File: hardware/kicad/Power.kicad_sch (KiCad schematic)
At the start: 0 parts

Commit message: start pwr circuitry
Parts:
- added C38: 4.7uF, Diode_SMD:D_SMF, symbol Device:C
- added C39: 10uF, Diode_SMD:D_SMF, symbol Device:C
- added C40: 100nF, Diode_SMD:D_SMF, symbol Device:C
- added D29: SMF5V0A, Diode_SMD:D_SMF, symbol Diode:SMF5V0A
- added F1: Polyfuse, Package_LCC:PLCC-84_29.3x29.3mm_P1.27mm, symbol Device:Polyfuse
- added FB2: FerriteBead, symbol Device:FerriteBead
- added H1, H2, H3, H4: MountingHole_Pad, Connector_Audio:Jack_6.35mm_Neutrik_NMJ6HFD2-AU_Horizontal, symbol Mechanical:MountingHole_Pad
- added U2: LP2985-5.0, Package_TO_SOT_SMD:SOT-23-5, symbol Regulator_Linear:LP2985-5.0
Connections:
- new net: C38.1, D29.1 (A1), F1.2, FB2.1
- new net GND: C38.2, C39.2, C40.2, D29.2 (A2)
- new net SHIELD_GND: H1.1, H2.1, H3.1, H4.1
- new net USB_VBUS: C39.1, C40.1, FB2.2
- new net VBUS_RAW: F1.1
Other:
- note added: "Analog 3.3V Conversion"
- note added: "Chassis/Shield GND Conn."
- note added: "Digital 3.3V Conversion"
- note added: "USB VBUS Entry"
- company: (none) -> Jeevan Sanchez
- title: (none) -> Power Circuitry

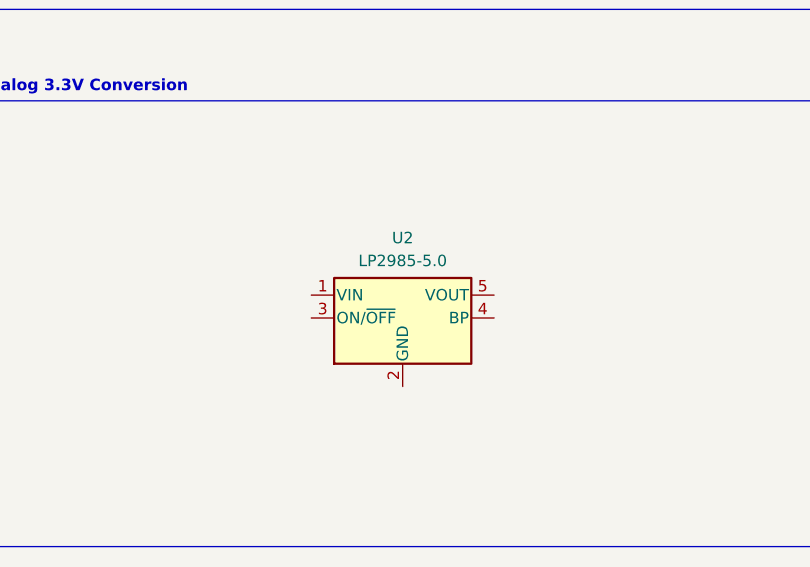
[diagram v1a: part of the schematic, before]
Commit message: ldo selection
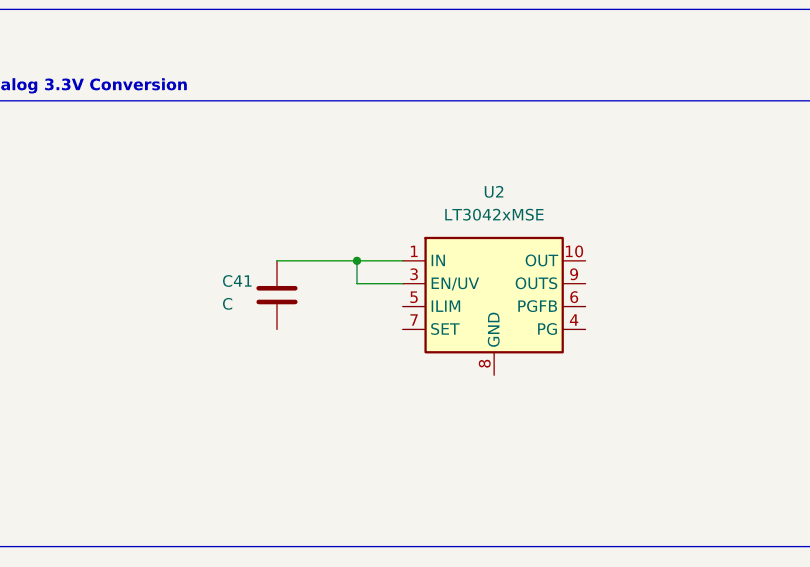
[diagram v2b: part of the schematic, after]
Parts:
- removed U2: LP2985-5.0, Package_TO_SOT_SMD:SOT-23-5, symbol Regulator_Linear:LP2985-5.0
- added C41: C, Package_SO:MSOP-10-1EP_3x3mm_P0.5mm_EP1.68x1.88mm, symbol Device:C
- added U2: LT3042xMSE, Package_SO:MSOP-10-1EP_3x3mm_P0.5mm_EP1.68x1.88mm, symbol Regulator_Linear:LT3042xMSE
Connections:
- new net: C41.1, U2.1 (IN), U2.2 (IN), U2.3 (EN/UV)
- new net: U2.11 (GND), U2.8 (GND)
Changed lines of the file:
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@@
 		(color 0 0 0 0)
 	)
+	(junction
+		(at 64.77 85.09)
+		(diameter 0)
+		(color 0 0 0 0)
+	)
+	(wire
+		(pts
+			(xy 55.88 85.09) (xy 64.77 85.09)
+		)
+		(stroke
+			(width 0)
+			(type default)
+		)
+	)
 	(wire
 		(pts
@@
 	(wire
 		(pts
+			(xy 64.77 85.09) (xy 69.85 85.09)
+		)
+		(stroke
+			(width 0)
+			(type default)
+		)
+	)
+	(wire
+		(pts
 			(xy 243.84 35.56) (xy 257.81 35.56)
 		)
@@
 		(pts
 			(xy 83.82 39.37) (xy 95.25 39.37)
+		)
+		(stroke
+			(width 0)
+			(type default)
+		)
+	)
+	(wire
+		(pts
+			(xy 69.85 87.63) (xy 64.77 87.63)
+		)
+		(stroke
+			(width 0)
+			(type default)
+		)
+	)
+	(wire
+		(pts
+			(xy 64.77 87.63) (xy 64.77 85.09)
 		)
 		(stroke
@@
 	)
 	(symbol
+		(lib_id "Regulator_Linear:LT3042xMSE")
+		(at 80.01 87.63 0)
+		(unit 1)
+		(body_style 1)
+		(exclude_from_sim no)
+		(in_bom yes)
+		(on_board yes)
+		(in_pos_files yes)
+		(dnp no)
+		(fields_autoplaced yes)
+		(property "Reference" "U2"
+			(at 80.01 77.47 0)
+			(show_name no)
+			(do_not_autoplace no)
+			(effects
+				(font
+					(size 1.27 1.27)
+				)
+			)
+		)
+		(property "Value" "LT3042xMSE"
+			(at 80.01 80.01 0)
+			(show_name no)
+			(do_not_autoplace no)
+			(effects
+				(font
+					(size 1.27 1.27)
+				)
+			)
+		)
+		(property "Footprint" "Package_SO:MSOP-10-1EP_3x3mm_P0.5mm_EP1.68x1.88mm"
+			(at 80.01 79.375 0)
+			(hide yes)
+			(show_name no)
+			(do_not_autoplace no)
+			(effects
+				(font
+					(size 1.27 1.27)
+				)
+			)
+		)
+		(property "Datasheet" "https://www.analog.com/media/en/technical-documentation/data-sheets/3042fb.pdf"
+			(at 80.01 87.63 0)
+			(hide yes)
+			(show_name no)
+			(do_not_autoplace no)
+			(effects
+				(font
+					(size 1.27 1.27)
+				)
+			)
+		)
+		(property "Description" "200mA, Adjustable, Ultralow Noise, Ultrahigh PSRR RF Linear Regulator, MSOP-10"
+			(at 80.01 87.63 0)
+			(hide yes)
+			(show_name no)
+			(do_not_autoplace no)
+			(effects
+				(font
+					(size 1.27 1.27)
+				)
+			)
+		)
+		(pin "1"
+		)
+		(pin "9"
+		)
+		(pin "10"
+		)
+		(pin "2"
+		)
+		(pin "11"
+		)
+		(pin "8"
+		)
+		(pin "3"
+		)
+		(pin "7"
+		)
+		(pin "5"
+		)
+		(pin "4"
+		)
+		(pin "6"
+		)
+		(instances
+			(project "vireo-lite"
+				(path "/61005c45-a979-4676-8d6b-817cd7f4616a/33b8941b-d741-4787-8ae4-4d148ad50e4b"
+					(reference "U2")
+					(unit 1)
+				)
+			)
+		)
+	)
+	(symbol
 		(lib_id "Mechanical:MountingHole_Pad")
 		(at 254 33.02 0)
@@
 	)
 	(symbol
-		(lib_id "Regulator_Linear:LP2985-5.0")
-		(at 69.85 91.44 0)
-		(unit 1)
-		(body_style 1)
-		(exclude_from_sim no)
-		(in_bom yes)
-		(on_board yes)
-		(in_pos_files yes)
-		(dnp no)
-		(fields_autoplaced yes)
-		(property "Reference" "U2"
-			(at 69.85 82.55 0)
-			(show_name no)
-			(do_not_autoplace no)
-			(effects
-				(font
-					(size 1.27 1.27)
-				)
-			)
-		)
-		(property "Value" "LP2985-5.0"
-			(at 69.85 85.09 0)
-			(show_name no)
-			(do_not_autoplace no)
-			(effects
-				(font
-					(size 1.27 1.27)
-				)
-			)
-		)
-		(property "Footprint" "Package_TO_SOT_SMD:SOT-23-5"
-			(at 69.85 83.185 0)
-			(hide yes)
-			(show_name no)
-			(do_not_autoplace no)
-			(effects
-				(font
-					(size 1.27 1.27)
-				)
-			)
-		)
-		(property "Datasheet" "http://www.ti.com/lit/ds/symlink/lp2985.pdf"
-			(at 69.85 91.44 0)
-			(hide yes)
-			(show_name no)
-			(do_not_autoplace no)
-			(effects
-				(font
-					(size 1.27 1.27)
-				)
-			)
-		)
-		(property "Description" "150mA 16V Low-noise Low-dropout Regulator With Shutdown, 5.0V output voltage, SOT-23-5"
-			(at 69.85 91.44 0)
-			(hide yes)
-			(show_name no)
-			(do_not_autoplace no)
-			(effects
-				(font
-					(size 1.27 1.27)
-				)
-			)
-		)
-		(pin "1"
-		)
-		(pin "4"
-		)
-		(pin "3"
-		)
-		(pin "2"
-		)
-		(pin "5"
-		)
-		(instances
-			(project "vireo-lite"
-				(path "/61005c45-a979-4676-8d6b-817cd7f4616a/33b8941b-d741-4787-8ae4-4d148ad50e4b"
-					(reference "U2")
-					(unit 1)
-				)
-			)
-		)
-	)
-	(symbol
 		(lib_id "Device:C")
 		(at 83.82 43.18 0)
@@
 					(unit 1)
 				)
+			)
+		)
+	)
+	(symbol
+		(lib_id "Device:C")
+		(at 55.88 88.9 0)
+		(unit 1)
+		(body_style 1)
+		(exclude_from_sim no)
+		(in_bom yes)
+		(on_board yes)
+		(in_pos_files yes)
+		(dnp no)
+		(property "Reference" "C41"
+			(at 49.784 87.376 0)
+			(show_name no)
+			(do_not_autoplace no)
+			(effects
+				(font
+					(size 1.27 1.27)
+				)
+				(justify left)
+			)
+		)
+		(property "Value" "C"
+			(at 49.784 89.916 0)
+			(show_name no)
+			(do_not_autoplace no)
+			(effects
+				(font
+					(size 1.27 1.27)
+				)
+				(justify left)
+			)
+		)
+		(property "Footprint" "Package_SO:MSOP-10-1EP_3x3mm_P0.5mm_EP1.68x1.88mm"
+			(at 56.8452 92.71 0)
+			(hide yes)
+			(show_name no)
+			(do_not_autoplace no)
+			(effects
+				(font
+					(size 1.27 1.27)
+				)
+			)
+		)
+		(property "Datasheet" ""
+			(at 55.88 88.9 0)
+			(hide yes)
+			(show_name no)
+			(do_not_autoplace no)
+			(effects
+				(font
+					(size 1.27 1.27)
+				)
+			)
+		)
+		(property "Description" "Unpolarized capacitor"
+			(at 55.88 88.9 0)
+			(hide yes)
+			(show_name no)
+			(do_not_autoplace no)
+			(effects
+				(font
+					(size 1.27 1.27)
+				)
+			)
+		)
+		(pin "1"
+		)
+		(pin "2"
+		)
+		(instances
+			(project "vireo-lite"
+				(path "/61005c45-a979-4676-8d6b-817cd7f4616a/33b8941b-d741-4787-8ae4-4d148ad50e4b"
+					(reference "C41")
+					(unit 1)
+				)
